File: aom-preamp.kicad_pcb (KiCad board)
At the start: 2 copper layers, 81 x 26.5 mm, 47 parts, among them J1 Battery_9V, J3 USB_B_Mini, J4 PJ-320B, Q1 BC849, Q2 BC859, Q3 BC859, Q4 BC859, Q5 BC849, U1 CM108B, U2 PC817

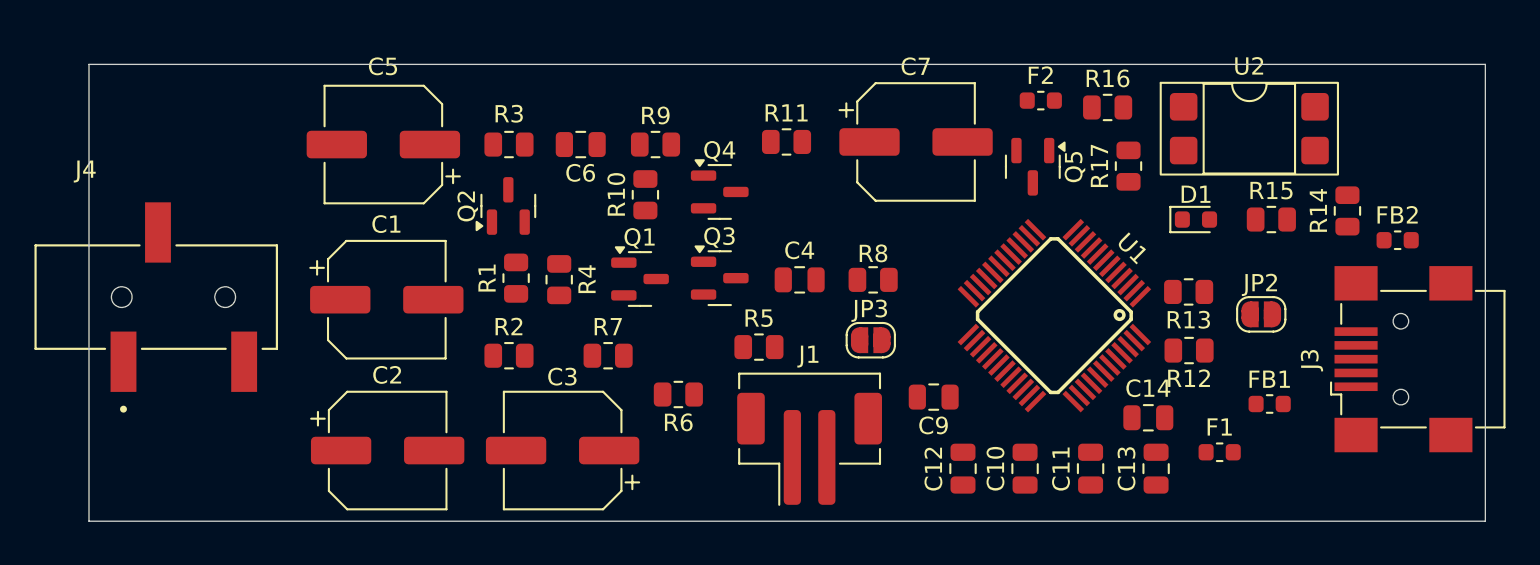
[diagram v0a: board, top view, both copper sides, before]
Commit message: update
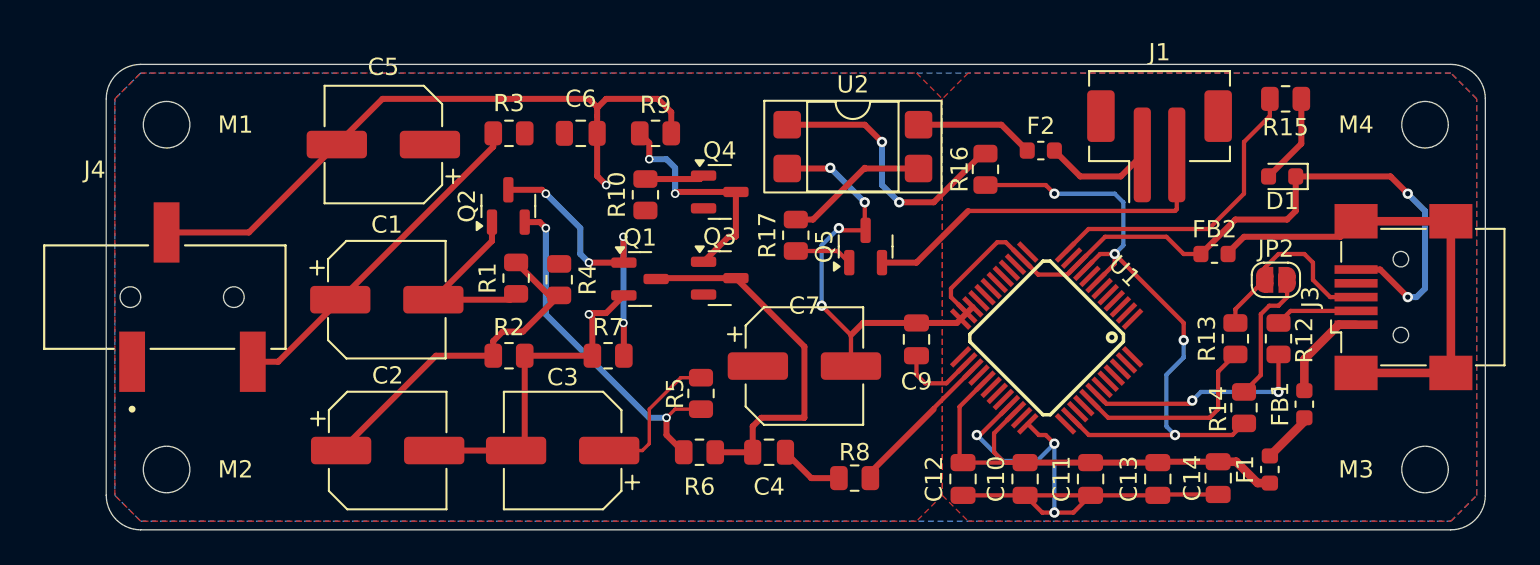
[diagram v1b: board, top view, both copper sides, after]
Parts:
- removed JP3: PullUp, Jumper:SolderJumper-2_P1.3mm_Open_RoundedPad1.0x1.5mm
- removed R11: 10R, Resistor_SMD:R_0805_2012Metric
- added M1: MountingHole_2.7mm_M2.5, MountingHole:MountingHole_2.7mm_M2.5, F.Cu at (95.5, 79.0)
- added M2: MountingHole_2.7mm_M2.5, MountingHole:MountingHole_2.7mm_M2.5, F.Cu at (95.5, 99.0)
- added M3: MountingHole_2.7mm_M2.5, MountingHole:MountingHole_2.7mm_M2.5, F.Cu at (168.5, 99.0)
- added M4: MountingHole_2.7mm_M2.5, MountingHole:MountingHole_2.7mm_M2.5, F.Cu at (168.5, 79.0)
- moved J1 26.8 mm to (153.1, 80.2)
- moved U2 23.0 mm to (135.3, 80.3)
- moved R17 19.7 mm to (132.0, 85.4)
- moved C7 14.5 mm to (132.5, 93.0)
- moved R14 12.9 mm to (158.0, 95.4)
- moved R8 11.6 mm to (135.4, 99.5)
- moved Q5 10.7 mm to (136.1, 86.1), turned to 90 degrees
- moved FB2 10.7 mm to (156.3, 86.5)
- moved C4 10.2 mm to (130.4, 98.0)
- moved R16 7.94 mm to (143.0, 81.6), turned to -90 degrees
- moved R15 7.05 mm to (160.4, 77.5), turned to 180 degrees
- moved D1 5.59 mm to (160.2, 82.0), turned to 180 degrees
- moved C14 5.35 mm to (156.5, 99.5), turned to -90 degrees
- moved R12 5.23 mm to (160.0, 91.4), turned to 90 degrees
- moved R5 4.30 mm to (126.5, 94.6), turned to 90 degrees
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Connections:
- C2 pad 2: GND1 -> GND
- C3 pad 2: GND1 -> GND
- C5 pad 1: Net-(Q4-E) -> 9V_BAT
- C5 pad 2: GND1 -> GND
- C6 pad 1: GND1 -> GND
- C6 pad 2: Net-(Q4-E) -> 9V_BAT
- C7 pad 2: GND1 -> GND
- J4 pad 2: GND1 -> GND
- Q1 pad 2: GND1 -> GND
- Q4 pad 2: Net-(Q4-E) -> 9V_BAT
- Q5 pad 3: GND1 -> GND
- R10 pad 1: Net-(Q4-E) -> 9V_BAT
- R2 pad 2: GND1 -> GND
- R3 pad 1: Net-(Q4-E) -> 9V_BAT
- R4 pad 1: Net-(Q4-E) -> 9V_BAT
- R7 pad 1: GND1 -> GND
- R9 pad 2: GND1 -> GND
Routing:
- net GND: track 0.00 -> 163.5 mm, vias 0 -> 11
- net V3.3: track 0.00 -> 39.4 mm, vias 0 -> 4
- net Net-(J3-Shield): track 0.00 -> 28.1 mm
- net AVDD1: track 0.00 -> 27.9 mm
- net 9V_GND: track 0.00 -> 21.5 mm
- net Net-(Q1-C): track 0.00 -> 21.3 mm
- net Net-(Q2-E): track 0.00 -> 20.5 mm, vias 0 -> 2
- net Net-(C2-Pad1): track 0.00 -> 20.2 mm
- net Net-(C1-Pad1): track 0.00 -> 19.9 mm
- net LEDO: track 0.00 -> 17.9 mm
- net Net-(Q1-B): track 0.00 -> 17.7 mm, vias 0 -> 4
- net Net-(R16-Pad1): track 0.00 -> 16.0 mm, vias 0 -> 2
- net Net-(Q3-B): track 0.00 -> 13.6 mm, vias 0 -> 2
- net Net-(R12-Pad1): track 0.00 -> 13.3 mm, vias 0 -> 2
- net Net-(R13-Pad1): track 0.00 -> 11.7 mm
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- added copper zone on F.Cu, net 9V_BAT
- added copper zone on B.Cu, net GND
- added copper zone on F.Cu, net V3.3
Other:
- board size 81 x 26.5 mm -> 80 x 27 mm
